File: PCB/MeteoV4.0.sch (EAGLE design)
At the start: 44 parts, among them IC1 MCP73832T, J1 POWER_JACKPTH

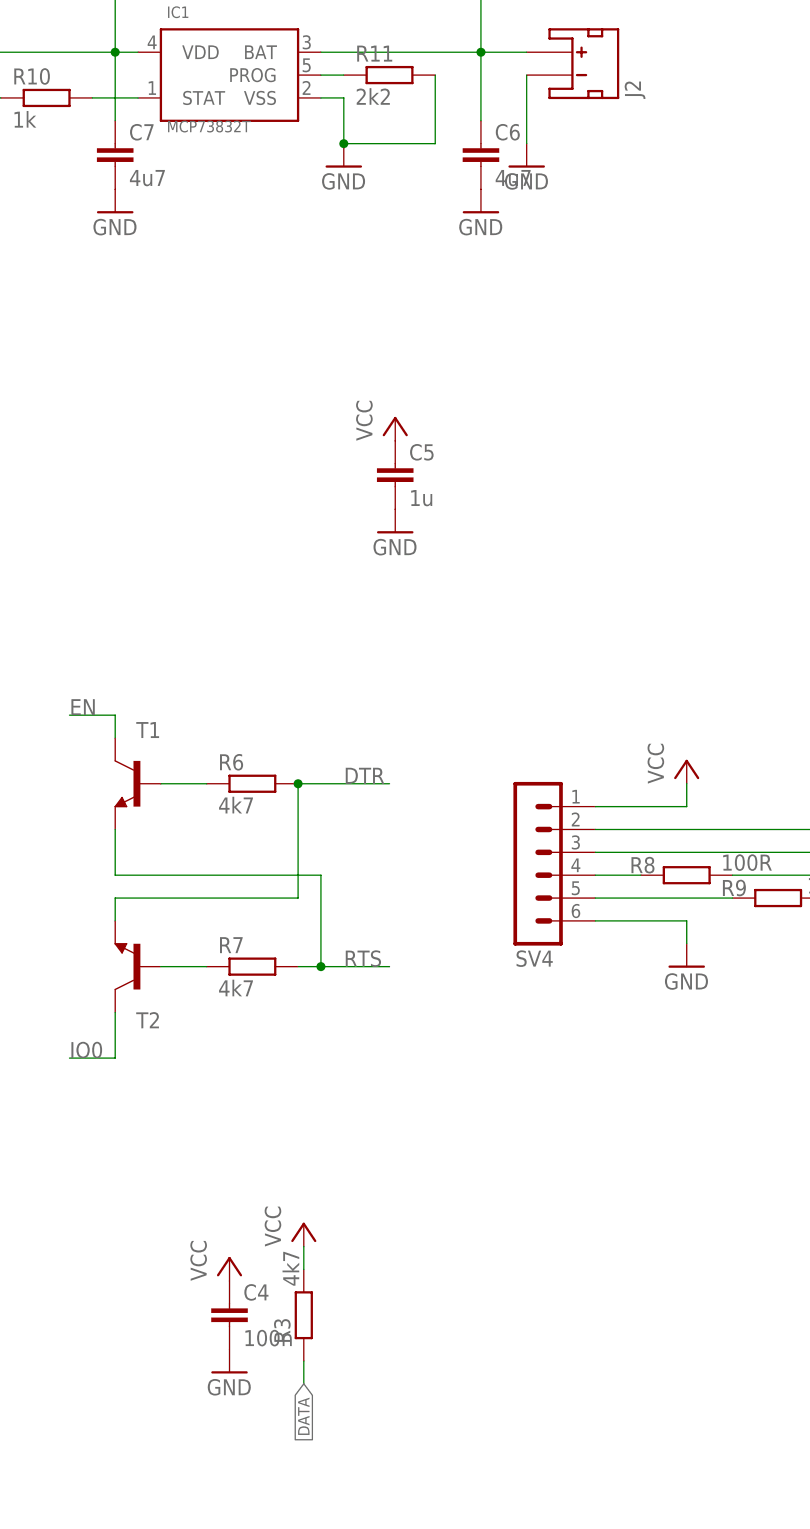
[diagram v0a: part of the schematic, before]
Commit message: Add files via upload
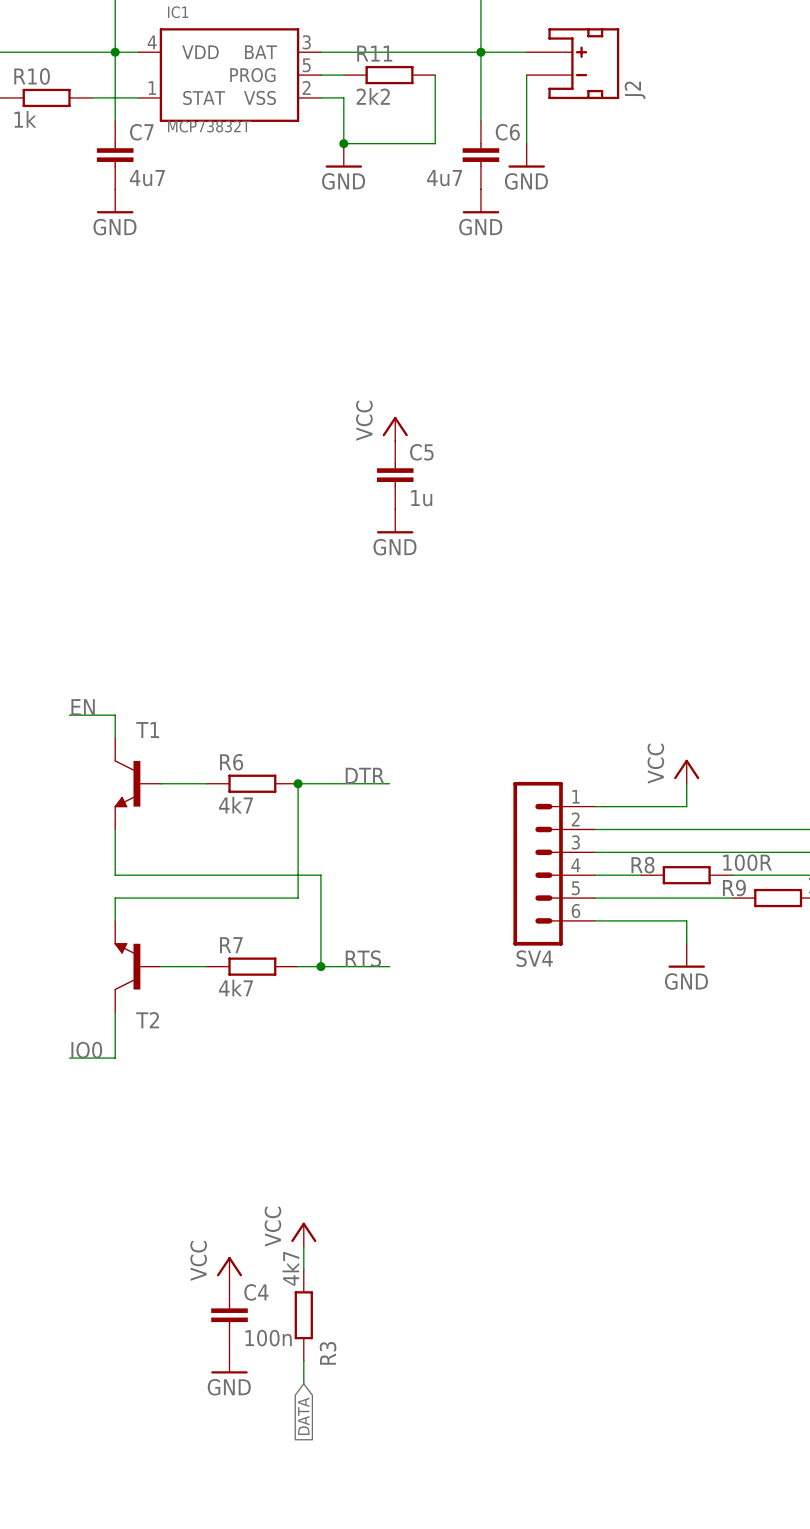
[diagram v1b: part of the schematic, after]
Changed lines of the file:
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@@
 </instance>
 <instance part="R3" gate="G$1" x="155.575" y="22.225" smashed="yes" rot="R90">
-<attribute name="NAME" x="154.0764" y="19.05" size="1.778" layer="95" rot="R90"/>
+<attribute name="NAME" x="159.1564" y="16.51" size="1.778" layer="95" rot="R90"/>
 <attribute name="VALUE" x="155.067" y="25.4" size="1.778" layer="96" rot="R90"/>
 </instance>
@@
 <instance part="C6" gate="G$1" x="175.26" y="152.4" smashed="yes">
 <attribute name="NAME" x="176.784" y="152.781" size="1.778" layer="95"/>
-<attribute name="VALUE" x="176.784" y="147.701" size="1.778" layer="96"/>
+<attribute name="VALUE" x="169.164" y="147.701" size="1.778" layer="96"/>
 </instance>
 <instance part="C7" gate="G$1" x="134.62" y="152.4" smashed="yes">
